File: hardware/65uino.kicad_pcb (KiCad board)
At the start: 2 copper layers, 75.2 x 53.5 mm, 50 parts, among them J1 Barrel_Jack_MountingPin, J2 USB_B_Micro, J3 OLED, SW1 RST, SW2 BTN, U1 R6507, U2 74HC04, U3 6532, U4 w27C512, U5 MIC5504-3.3YM5, U6 LM1117-5.0, X1 NC, Y1 1Mhz

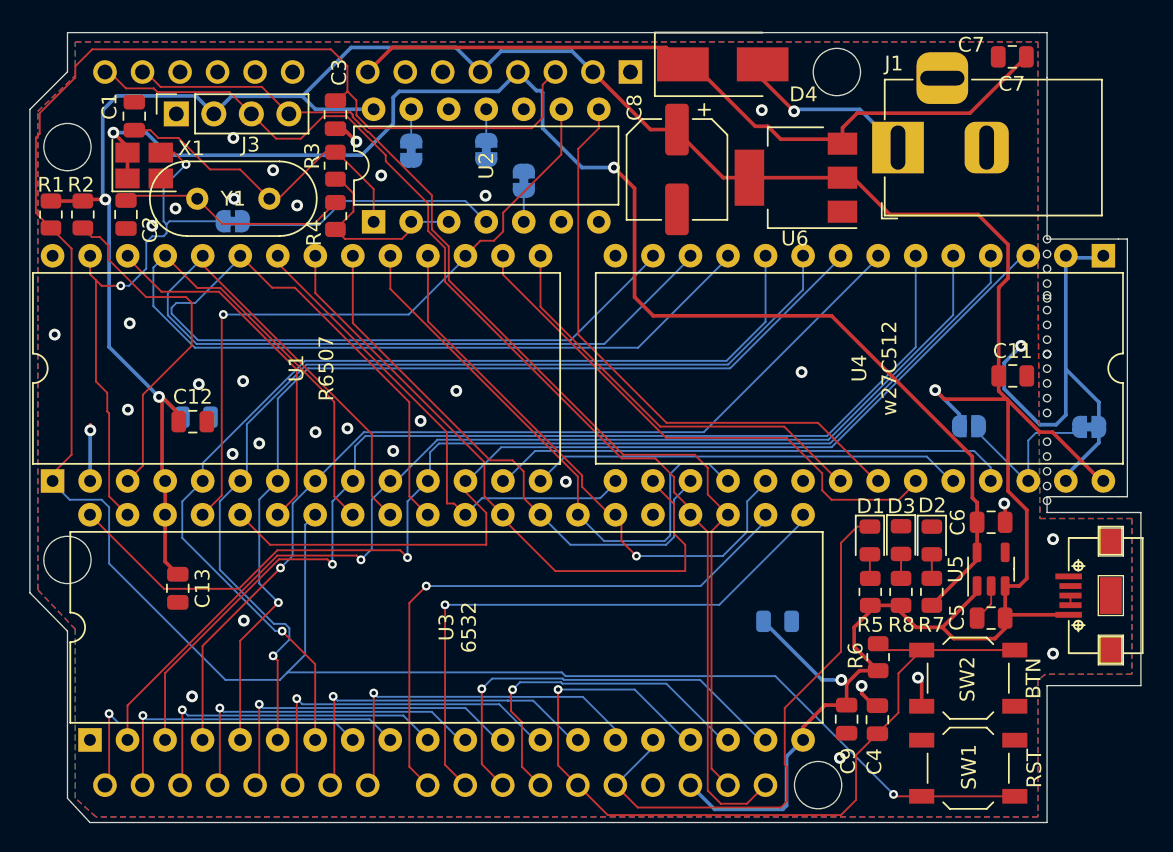
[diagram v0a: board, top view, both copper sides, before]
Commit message: 68.6mm
Edge cuts
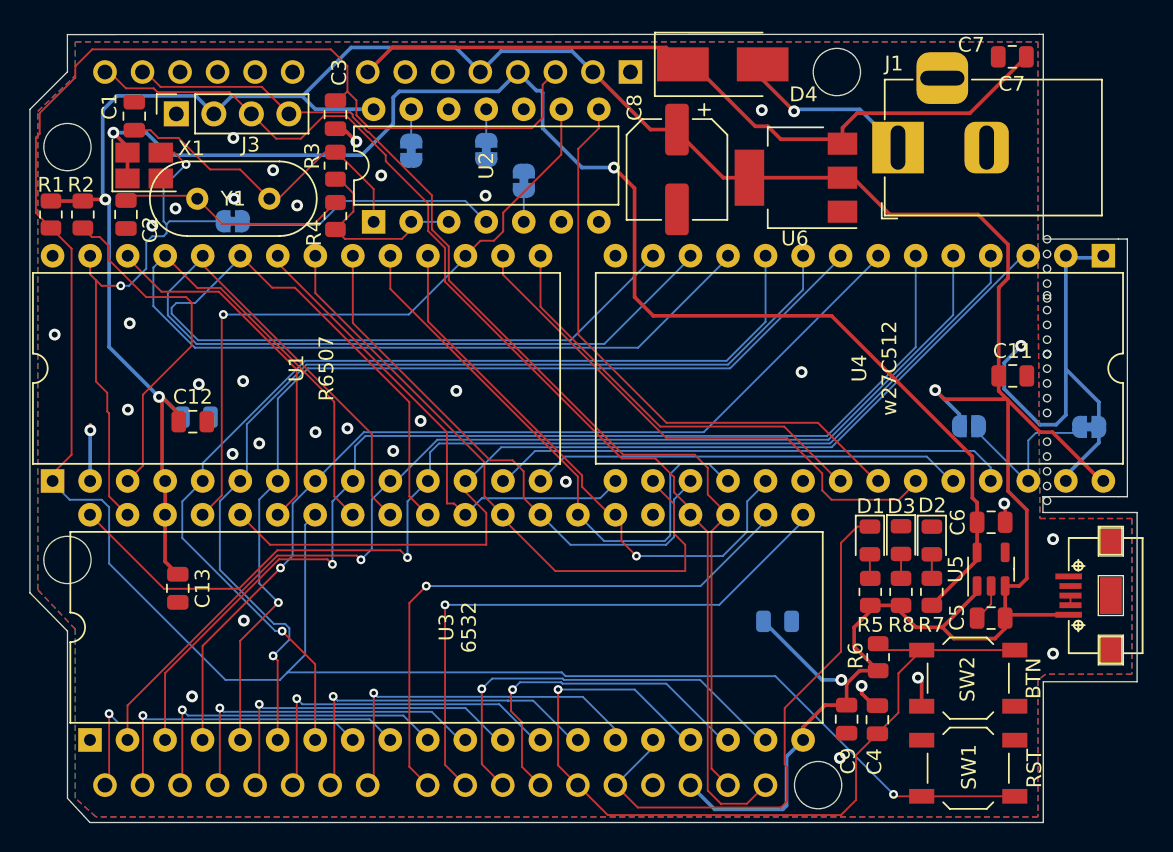
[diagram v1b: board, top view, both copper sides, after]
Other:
- board size 75.2 x 53.5 mm -> 74.9 x 53.3 mm
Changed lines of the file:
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@@
   (gr_line (start 117.2972 95.5802) (end 118.618 94.107) (layer "B.SilkS") (width 0.1))
   (gr_line (start 175.6156 79.8068) (end 176.2252 79.8068) (layer "Edge.Cuts") (width 0.05))
-  (gr_line (start 170.7896 92.5932) (end 170.7896 101.854) (layer "Edge.Cuts") (width 0.05))
+  (gr_line (start 170.5356 92.329) (end 170.5356 101.854) (layer "Edge.Cuts") (width 0.05))
   (gr_line (start 104.4956 100.2132) (end 104.4956 88.9) (layer "Edge.Cuts") (width 0.05))
-  (gr_line (start 170.7896 60.8432) (end 170.7896 62.3672) (layer "Edge.Cuts") (width 0.05))
-  (gr_line (start 170.2816 48.3972) (end 170.7896 48.3972) (layer "Edge.Cuts") (width 0.05))
+  (gr_line (start 170.5356 60.8432) (end 170.5356 62.3672) (layer "Edge.Cuts") (width 0.05))
+  (gr_line (start 170.2816 48.514) (end 170.5356 48.514) (layer "Edge.Cuts") (width 0.05))
   (gr_line (start 101.9556 53.594) (end 104.4956 51.054) (layer "Edge.Cuts") (width 0.05))
-  (gr_line (start 177.1396 80.8736) (end 170.7896 80.8736) (layer "Edge.Cuts") (width 0.05))
+  (gr_line (start 176.8856 80.8736) (end 170.5102 80.8736) (layer "Edge.Cuts") (width 0.05))
   (gr_line (start 101.9556 86.3092) (end 101.9556 53.594) (layer "Edge.Cuts") (width 0.05))
-  (gr_line (start 104.4956 48.3972) (end 170.2816 48.3972) (layer "Edge.Cuts") (width 0.05))
-  (gr_line (start 170.7896 48.3972) (end 170.7896 51.4452) (layer "Edge.Cuts") (width 0.05))
+  (gr_line (start 104.49 48.53) (end 170.2816 48.514) (layer "Edge.Cuts") (width 0.05))
+  (gr_line (start 170.5356 48.514) (end 170.5356 51.6382) (layer "Edge.Cuts") (width 0.05))
   (gr_line (start 106.0196 101.854) (end 104.4956 100.2132) (layer "Edge.Cuts") (width 0.05))
   (gr_line (start 104.4956 88.9) (end 101.9556 86.3092) (layer "Edge.Cuts") (width 0.05))
-  (gr_line (start 175.6156 79.8068) (end 170.7896 79.8068) (layer "Edge.Cuts") (width 0.05))
-  (gr_line (start 104.4956 51.054) (end 104.4956 48.3972) (layer "Edge.Cuts") (width 0.05))
+  (gr_line (start 175.6156 79.8068) (end 170.5102 79.8068) (layer "Edge.Cuts") (width 0.05))
+  (gr_line (start 104.4956 51.054) (end 104.49 48.53) (layer "Edge.Cuts") (width 0.05))
   (gr_line (start 175.6156 62.3672) (end 176.2252 62.3672) (layer "Edge.Cuts") (width 0.05))
   (gr_line (start 170.5356 101.854) (end 106.0196 101.854) (layer "Edge.Cuts") (width 0.05))
-  (gr_line (start 177.1396 92.5932) (end 177.1396 80.8736) (layer "Edge.Cuts") (width 0.05))
-  (gr_line (start 170.7896 60.8432) (end 170.7896 51.4452) (layer "Edge.Cuts") (width 0.05))
+  (gr_line (start 176.8856 92.329) (end 176.8856 80.8736) (layer "Edge.Cuts") (width 0.05))
+  (gr_line (start 170.5356 60.8432) (end 170.5356 51.6382) (layer "Edge.Cuts") (width 0.05))
   (gr_line (start 176.2252 62.3672) (end 176.2252 79.8068) (layer "Edge.Cuts") (width 0.05))
-  (gr_line (start 170.7896 79.8068) (end 170.7896 80.8736) (layer "Edge.Cuts") (width 0.05))
-  (gr_line (start 170.7896 92.5932) (end 177.1396 92.5932) (layer "Edge.Cuts") (width 0.05))
-  (gr_line (start 170.7896 62.3672) (end 175.6156 62.3672) (layer "Edge.Cuts") (width 0.05))
-  (gr_line (start 170.5356 101.854) (end 170.7896 101.854) (layer "Edge.Cuts") (width 0.05))
+  (gr_line (start 170.5102 79.8068) (end 170.5102 80.8736) (layer "Edge.Cuts") (width 0.05))
+  (gr_line (start 170.5356 92.329) (end 176.8856 92.329) (layer "Edge.Cuts") (width 0.05))
+  (gr_line (start 170.5356 62.3672) (end 175.6156 62.3672) (layer "Edge.Cuts") (width 0.05))
+  (gr_line (start 170.5356 101.854) (end 170.5356 101.854) (layer "Edge.Cuts") (width 0.05))
   (gr_text "PA1\nD1\nTX" (at 110.8964 91.0844) (layer "B.SilkS")
     (effects (font (size 0.8 0.8) (thickness 0.13)) (justify mirror))
